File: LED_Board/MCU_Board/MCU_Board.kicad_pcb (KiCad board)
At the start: 2 copper layers, 39 x 39 mm, 30 parts, among them J1 Conn_01x01, J10 Conn_01x01, J11 Conn_01x01, J12 Conn_01x01, J13 Conn_01x01, J14 Conn_01x01, J15 Conn_01x01, J16 Conn_01x04, J2 Conn_01x01, J3 Conn_01x01, J4 Conn_01x04, J5 USB_B_Micro, J6 Conn_01x02, J7 Conn_01x01, J8 Conn_01x01, J9 Conn_01x01, U1 EL817, U2 ATtiny85-20SU

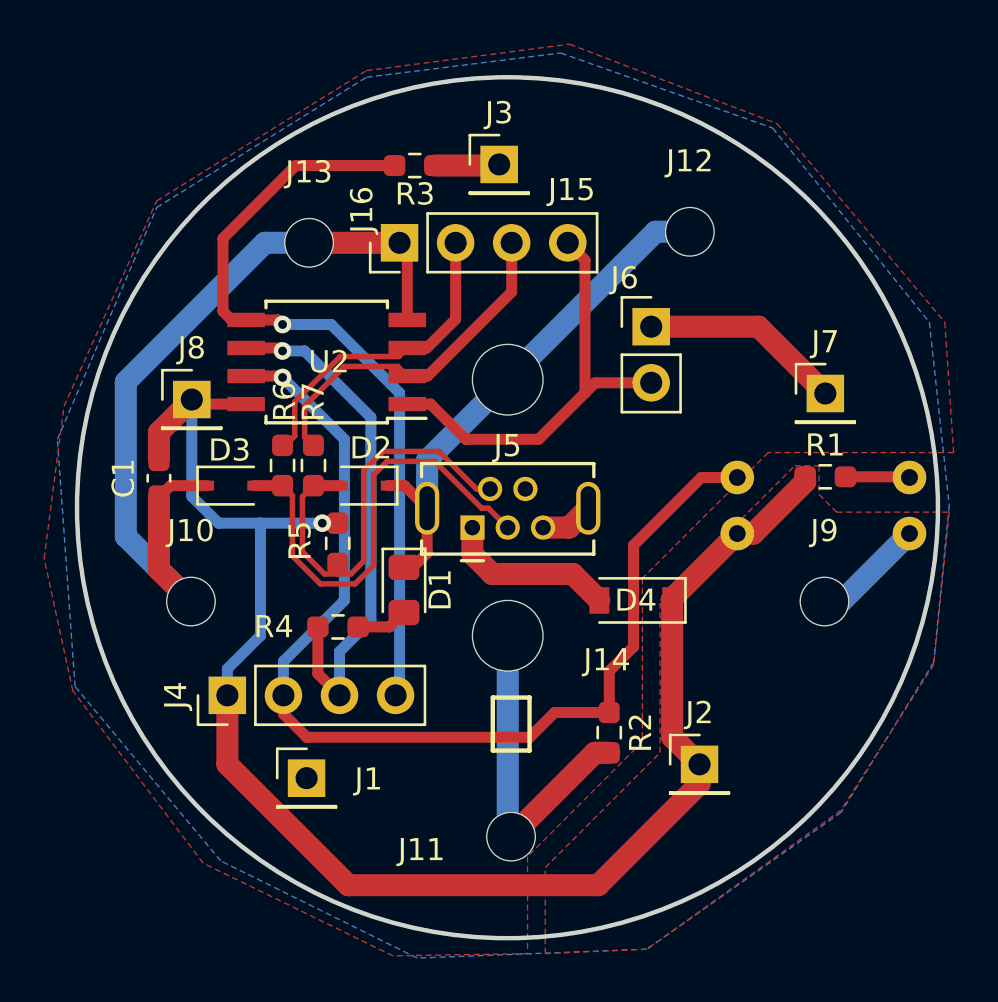
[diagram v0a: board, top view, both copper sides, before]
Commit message: Add files via upload
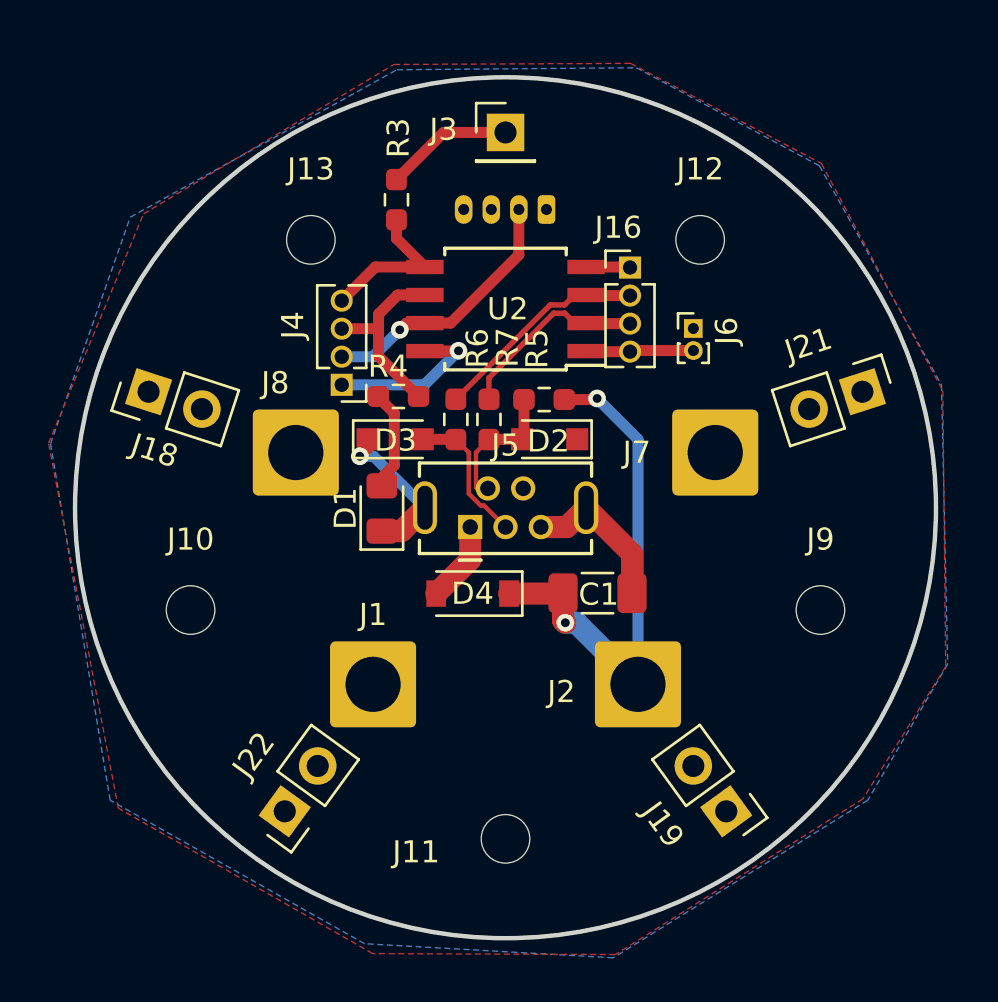
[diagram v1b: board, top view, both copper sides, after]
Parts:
- removed J14, J15: Conn_01x01, MountingHole:MountingHole_3.2mm_M3
- removed R1: 100, Resistor_SMD:R_0603_1608Metric_Pad0.98x0.95mm_HandSolder
- removed R2: 10K, Resistor_SMD:R_0603_1608Metric_Pad0.98x0.95mm_HandSolder
- removed U1: EL817, MCU_Board:Vishay_TCST1103
- added J18: Conn_01x02, Connector_PinHeader_2.54mm:PinHeader_1x02_P2.54mm_Vertical, F.Cu at (83.8, 94.7)
- added J19: Conn_01x02, Connector_PinHeader_2.54mm:PinHeader_1x02_P2.54mm_Vertical, F.Cu at (110.0, 113.8)
- added J20: Conn_01x04, Connector_Molex:Molex_PicoBlade_53047-0410_1x04_P1.25mm_Vertical, B.Cu at (101.9, 86.5)
- added J21: Conn_01x02, Connector_PinHeader_2.54mm:PinHeader_1x02_P2.54mm_Vertical, F.Cu at (116.2, 94.7)
- added J22: Conn_01x02, Connector_PinHeader_2.54mm:PinHeader_1x02_P2.54mm_Vertical, F.Cu at (90.0, 113.8)
- C1: footprint Capacitor_SMD:C_0603_1608Metric_Pad1.08x0.95mm_HandSolder -> Capacitor_SMD:C_1206_3216Metric_Pad1.33x1.80mm_HandSolder
- D2, D3: footprint Diode_SMD:D_SOD-323 -> Diode_SMD:D_SOD-323_HandSoldering
- J1, J2, J7, J8: footprint Connector_PinHeader_2.54mm:PinHeader_1x01_P2.54mm_Vertical -> Connector_Wire:SolderWire-2sqmm_1x01_D2mm_OD3.9mm
- J16, J4: footprint Connector_PinHeader_2.54mm:PinHeader_1x04_P2.54mm_Vertical -> Connector_PinHeader_1.27mm:PinHeader_1x04_P1.27mm_Vertical
- J6: footprint Connector_PinHeader_2.54mm:PinHeader_1x02_P2.54mm_Vertical -> Connector_PinHeader_1.00mm:PinHeader_1x02_P1.00mm_Vertical
- moved C1 20.5 mm to (104.2, 103.9), turned to 0 degrees
- moved J4 15.0 mm to (92.6, 94.4), turned to 180 degrees
- moved R5 11.4 mm to (101.8, 95.1), turned to 180 degrees
- moved R4 10.8 mm to (95.2, 95.0), turned to 0 degrees
- moved J16 10.5 mm to (105.6, 89.1), turned to 0 degrees
- moved D2 8.66 mm to (102.0, 96.9)
- moved U2 8.45 mm to (100.0, 91.0)
- moved R7 8.22 mm to (99.2, 96.0)
- moved R6 8.12 mm to (97.8, 96.0)
- moved D3 7.74 mm to (95.0, 96.9)
- moved D4 7.40 mm to (98.5, 103.9)
- moved J7 5.66 mm to (109.5, 97.5)
- moved J8 5.29 mm to (90.5, 97.5)
- moved J1 5.21 mm to (94.0, 108.0)
- moved J2 4.57 mm to (106.0, 108.0)
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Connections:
- net B3 renamed USB_N
- net B4 renamed USB_P
- net Net-(D2-Pad2) renamed /D_N
- net Net-(D3-Pad2) renamed /D_P
- J5 pad 4: Net-(J5-Pad4) -> unconnected-(J5-Pad4)
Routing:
- net GND: track 93.4 -> 16.4 mm, vias 0 -> 1
- net +5V: track 71.8 -> 31.0 mm, vias 1 -> 3
- net B2: track 48.9 -> 12.0 mm
- net B0: track 35.7 -> 7.07 mm, vias 1 -> 0
- net RESET: track 19.9 -> 4.89 mm
- net B1: track 23.6 -> 8.67 mm, vias 1 -> 0
- net /D_P: track 20.9 -> 6.49 mm
- net /D_N: track 19.3 -> 7.56 mm
- net USB_N: track 16.1 -> 8.77 mm
- net USB_P: track 14.6 -> 9.86 mm
- net VBUS: track 7.82 -> 3.65 mm
- net Net-(R1-Pad2): track 2.91 -> 0.00 mm
- net Net-(J3-Pad1): track 2.93 -> 5.83 mm
- net Net-(D1-Pad2): track 2.34 -> 4.58 mm
- added copper zone on B.Cu, net +5V
- removed copper zone on F.Cu, net +5V
- removed copper zone on B.Cu, net GND
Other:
- net class Default removed
